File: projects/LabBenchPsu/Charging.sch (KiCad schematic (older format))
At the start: 18 parts

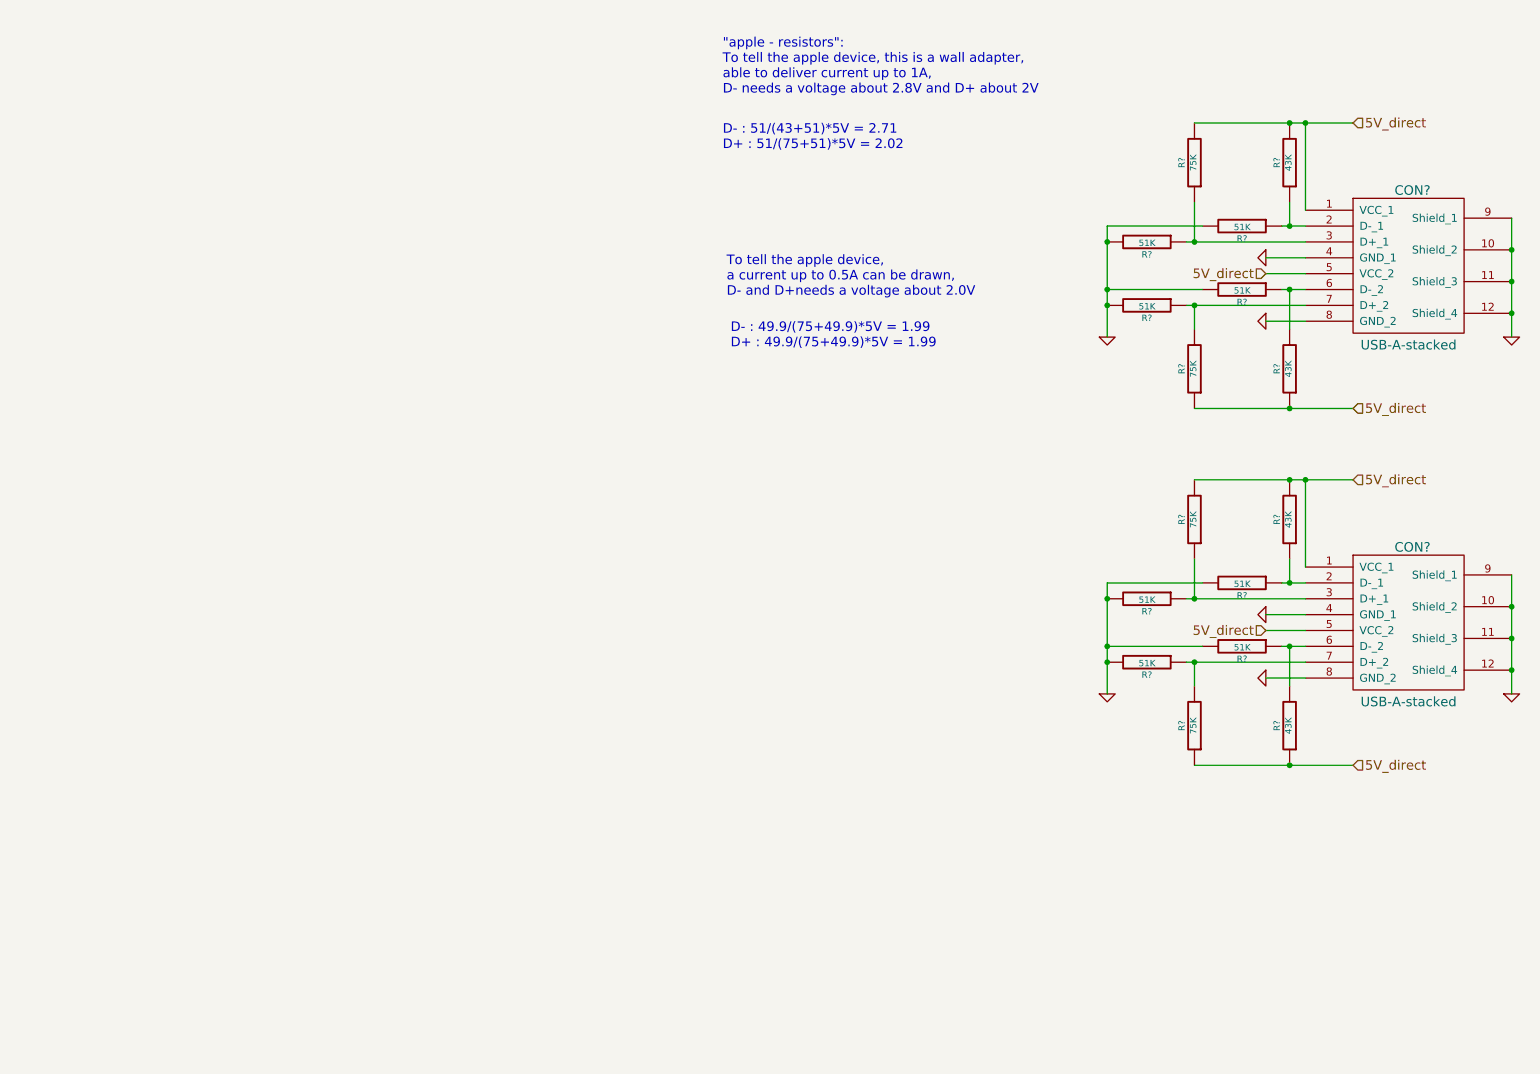
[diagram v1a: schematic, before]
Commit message: LabBenchPsu updated
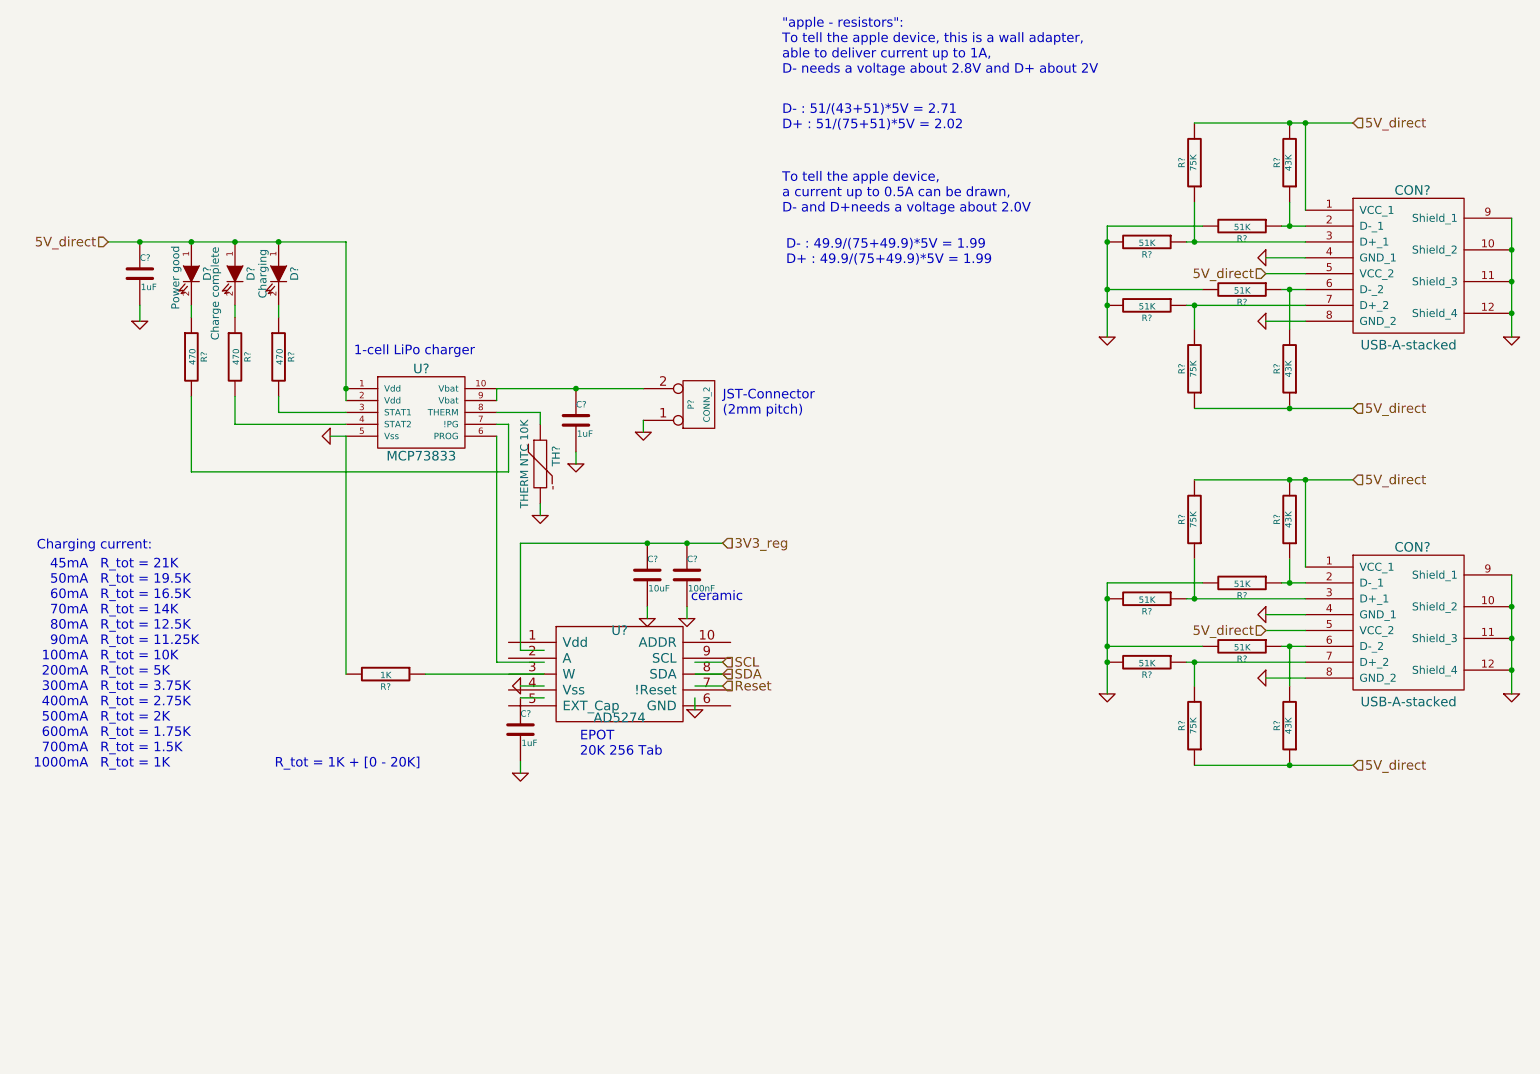
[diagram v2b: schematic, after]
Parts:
- added C? (x3): 1uF, symbol C
- added C?: 100nF, symbol C
- added C?: 10uF, symbol C
- added D?: Power good, symbol LED
- added D?: Charge complete, symbol LED
- added D?: Charging, symbol LED
- added P?: CONN_2, symbol CONN_2
- added R? (x3): 470, symbol R
- added R?: 1K, symbol R
- added TH?: THERM NTC 10K, symbol THERMISTOR
- added U?: AD5274, symbol AD5274
- added U?: MCP73833, symbol MCP73833
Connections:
- net labels added: 3V3_reg, Reset, SCL, SDA
- wire segments 36 -> 74
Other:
- note added: "1-cell LiPo charger"
- note added: "45mA\n50mA\n60mA\n70mA\n80mA\n90mA\n100mA\n200mA\n300mA\n400mA\n500mA\n600mA\n700mA\n1000mA"
- note added: "Charging current:\n"
- note added: "EPOT\n20K 256 Tab"
- note added: "JST-Connector\n(2mm pitch)"
- note added: "R_tot = 1K + [0 - 20K]"
- note added: "R_tot = 21K\nR_tot = 19.5K\nR_tot = 16.5K\nR_tot = 14K\nR_tot = 12.5K\nR_tot = 11.25K\nR_tot = 10K\nR_tot = 5K\nR_tot = 3.75K\nR_tot = 2.75K\nR_tot = 2K\nR_tot = 1.75K\nR_tot = 1.5K\nR_tot = 1K"
- note added: "ceramic"

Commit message: update LabBenchPsu
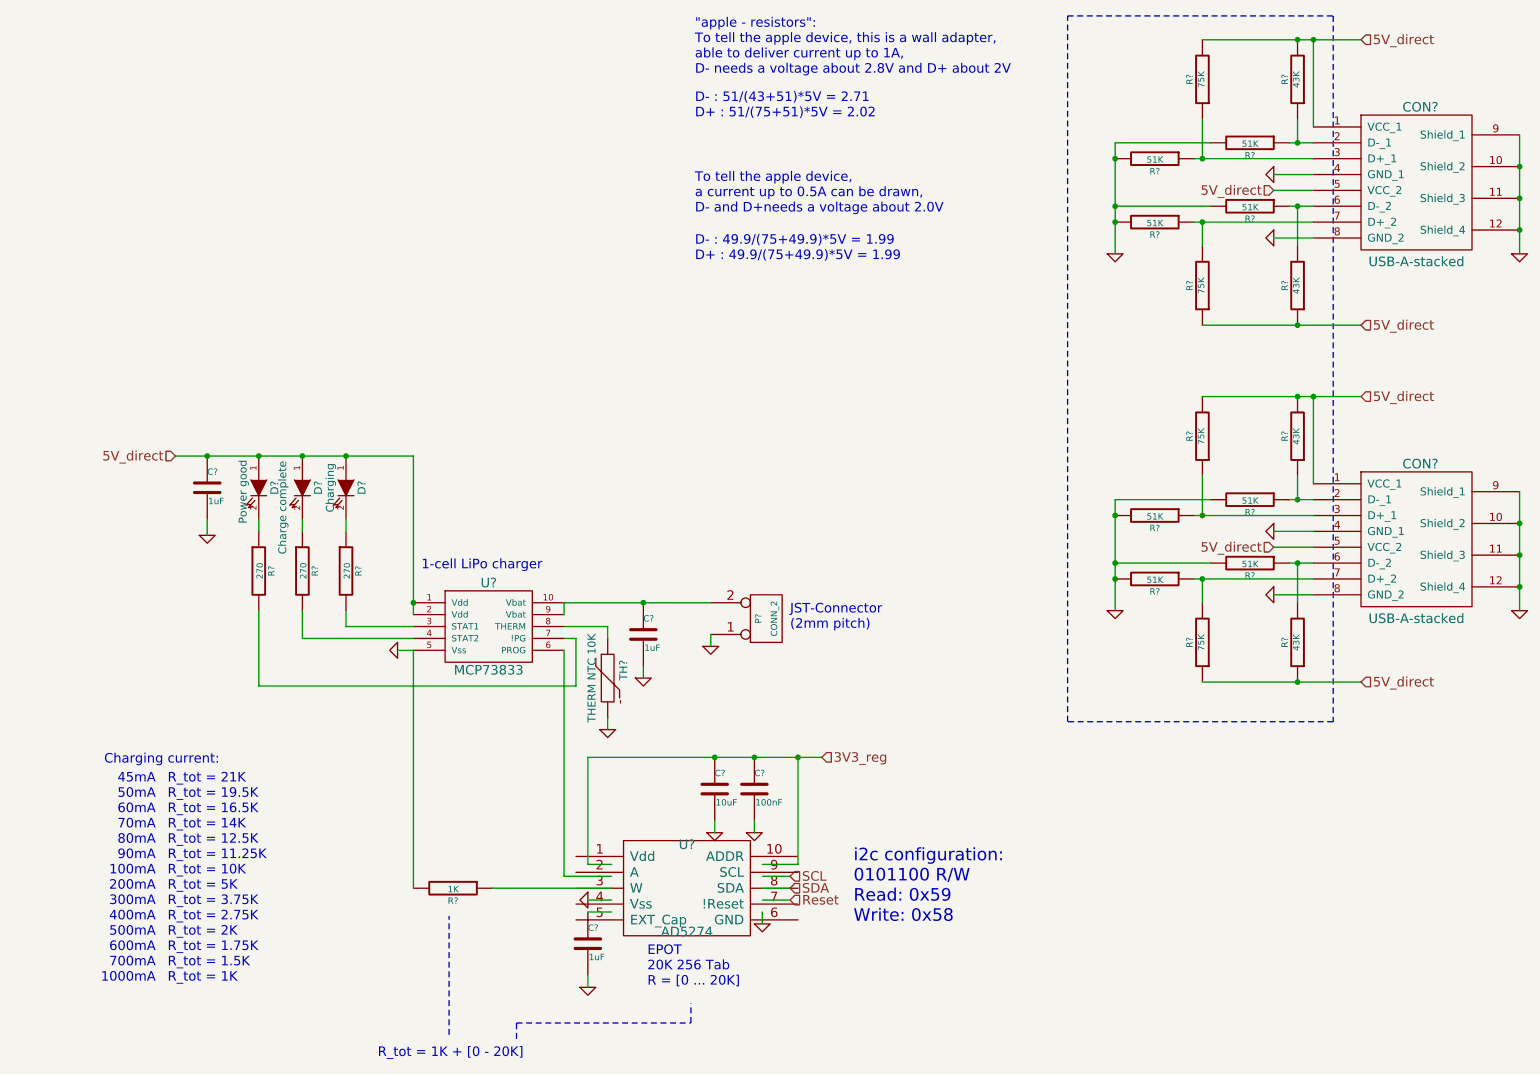
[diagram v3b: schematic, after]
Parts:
- R? (x3): value 470 -> 270
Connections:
- wire segments 74 -> 76
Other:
- note added: "EPOT\n20K 256 Tab\nR = [0 ... 20K]"
- note added: "i2c configuration:\n0101100 R/W\nRead: 0x59\nWrite: 0x58"
- note removed: "EPOT\n20K 256 Tab"
- note removed: "ceramic"
- moved on the sheet: C?, CON?, D?, P?, R?, TH?, U?

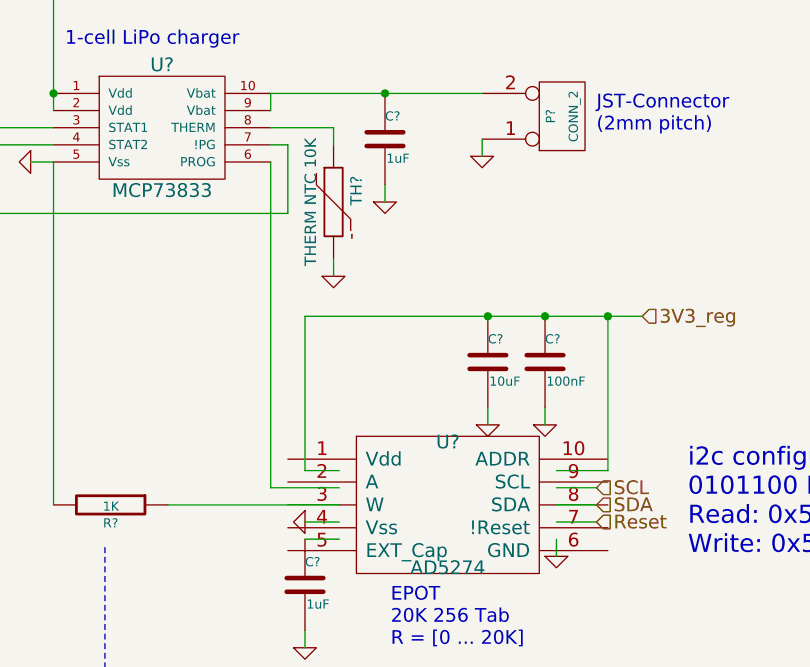
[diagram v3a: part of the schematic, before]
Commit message: small changes
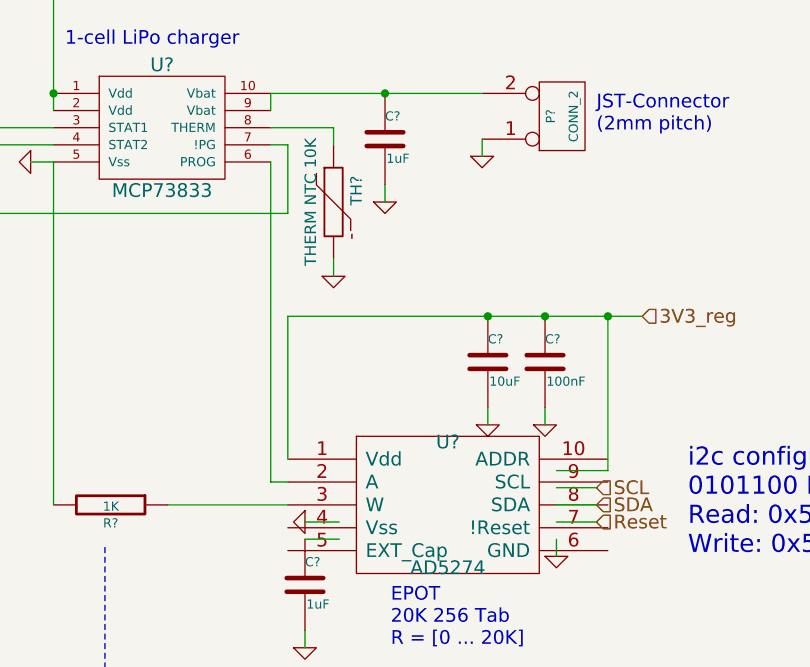
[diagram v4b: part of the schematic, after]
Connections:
- wire segments 76 -> 75
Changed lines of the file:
@@
 Wire Wire Line
 	3125 4875 3125 6375
-Wire Wire Line
-	4075 4875 4075 6300
 Text HLabel 5700 5550 2    60   Input ~ 0
 3V3_reg
@@
 $EndComp
 Wire Wire Line
-	3625 6375 4375 6375
-Wire Wire Line
-	4075 6300 4375 6300
-Wire Wire Line
-	4225 5550 5700 5550
+	4150 5550 5700 5550
 Connection ~ 5275 5550
-Wire Wire Line
-	4225 5550 4225 6225
-Wire Wire Line
-	4225 6225 4375 6225
 Connection ~ 5025 5550
 $Comp
@@
 	5550 6225 5550 5550
 Connection ~ 5550 5550
+Wire Wire Line
+	3625 6375 4150 6375
+Wire Wire Line
+	4075 4875 4075 6275
+Wire Wire Line
+	4075 6275 4150 6275
+Wire Wire Line
+	4150 5550 4150 6175
 $EndSCHEMATC
